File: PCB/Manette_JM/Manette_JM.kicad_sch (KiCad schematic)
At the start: 33 parts, among them J1 Jack 1, J10 Bouton 2, J11 Bouton 3, J12 Bouton 4, J13 DEL PWR, J14 Joystick 0, J15 Jack 7, J16 Jack 8, J2 Jack 3, J3 Jack 4, J4 Jack 5, J5 Jack 6, J6 Jack 2, J7 Jack 0, J8 Bouton 0, J9 Bouton 1, U1 NodeMCU1.0(ESP-12E), U2 ProMicro

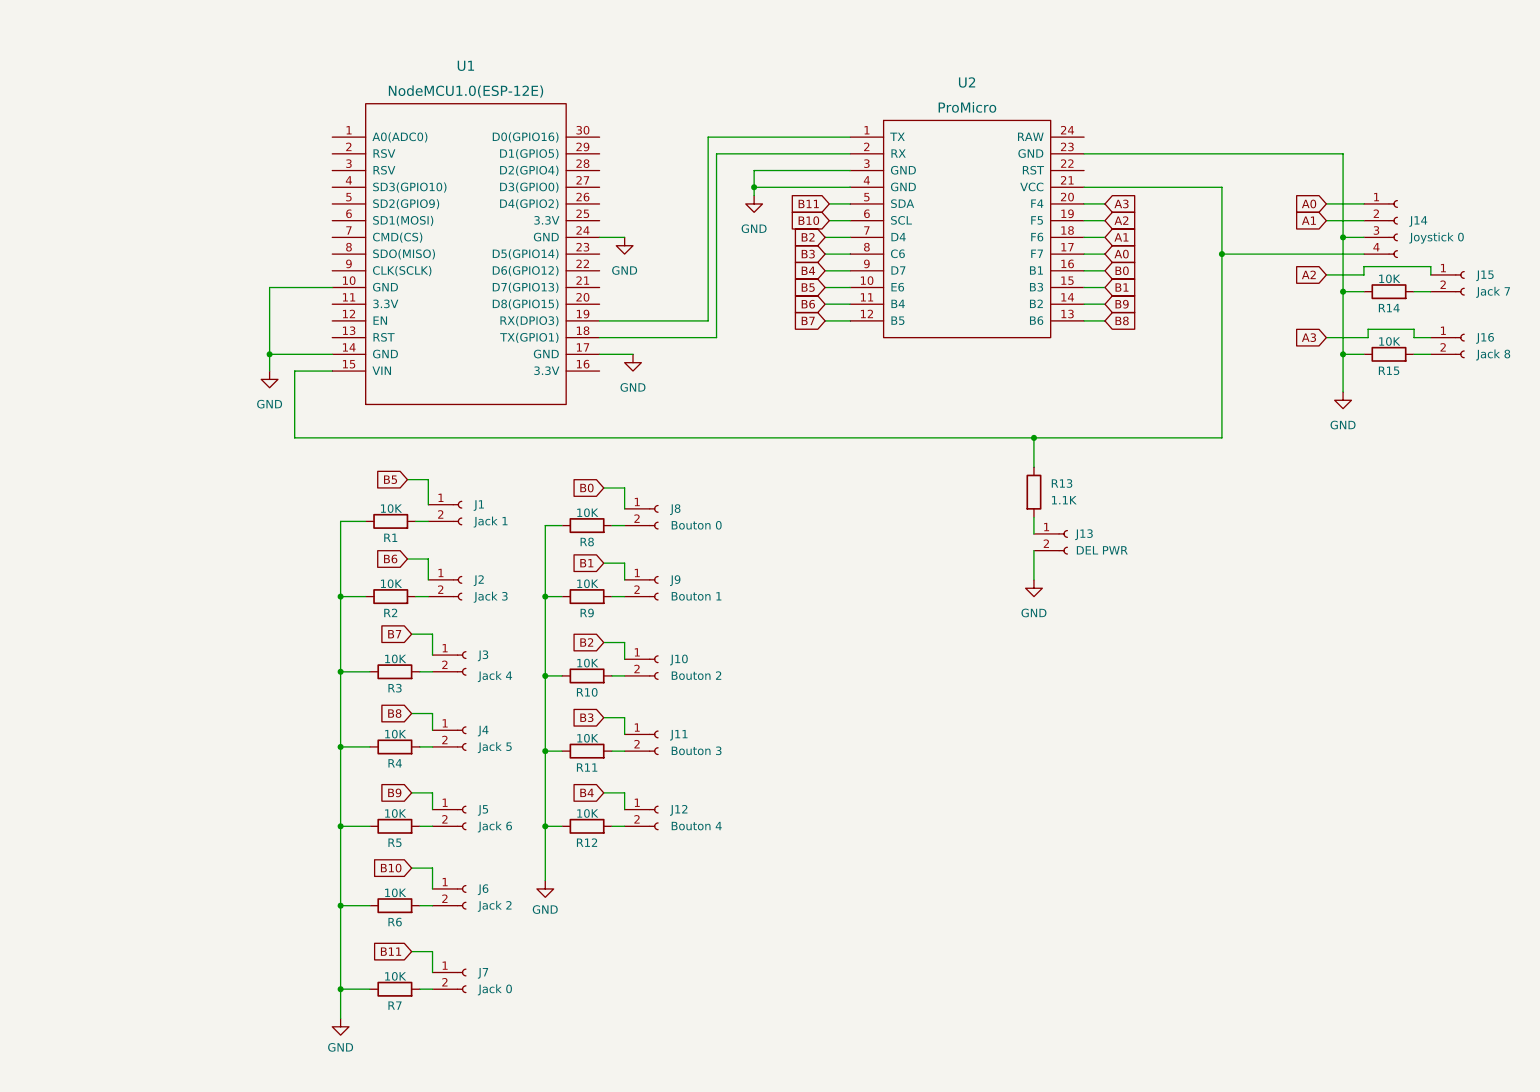
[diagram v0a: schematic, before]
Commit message: Quick changes
modification code et schéma
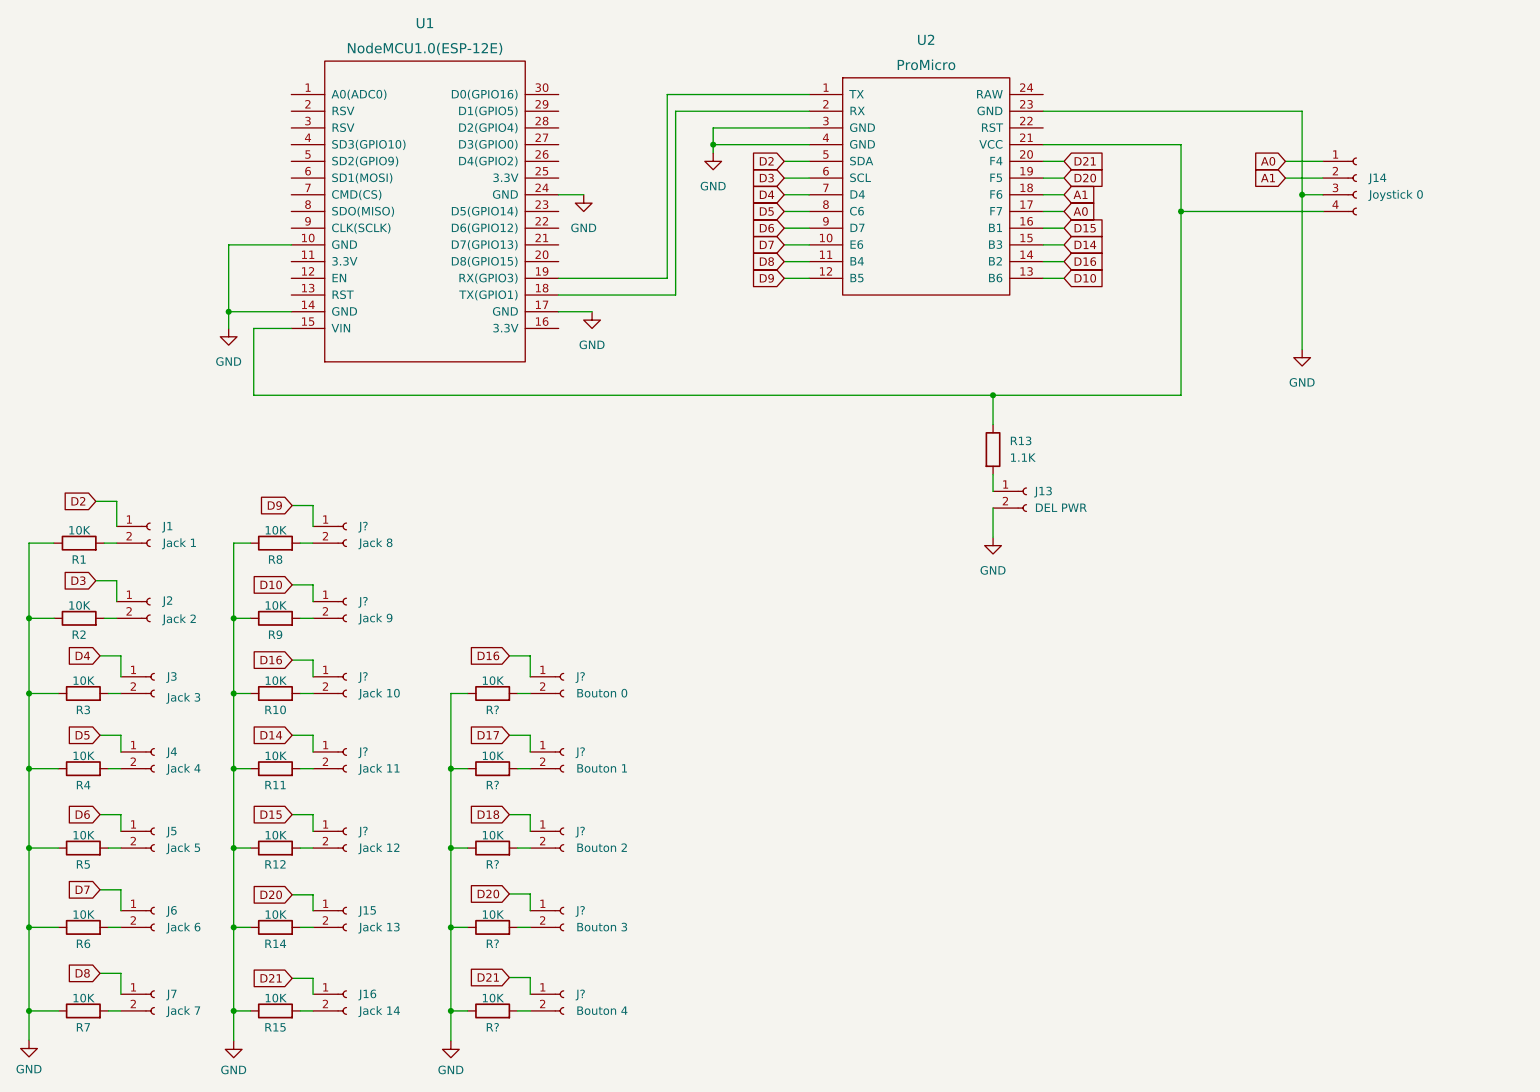
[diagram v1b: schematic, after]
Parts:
- removed J10: Bouton 2, Connector_PinHeader_2.54mm:PinHeader_1x02_P2.54mm_Vertical, symbol Connector:Conn_01x02_Female
- removed J11: Bouton 3, Connector_PinHeader_2.54mm:PinHeader_1x02_P2.54mm_Vertical, symbol Connector:Conn_01x02_Female
- removed J12: Bouton 4, Connector_PinHeader_2.54mm:PinHeader_1x02_P2.54mm_Vertical, symbol Connector:Conn_01x02_Female
- removed J8: Bouton 0, Connector_PinHeader_2.54mm:PinHeader_1x02_P2.54mm_Vertical, symbol Connector:Conn_01x02_Female
- removed J9: Bouton 1, Connector_PinHeader_2.54mm:PinHeader_1x02_P2.54mm_Vertical, symbol Connector:Conn_01x02_Female
- added J?: Bouton 1, Connector_PinHeader_2.54mm:PinHeader_1x02_P2.54mm_Vertical, symbol Connector:Conn_01x02_Female
- added J?: Bouton 4, Connector_PinHeader_2.54mm:PinHeader_1x02_P2.54mm_Vertical, symbol Connector:Conn_01x02_Female
- added J?: Jack 12, Connector_PinHeader_2.54mm:PinHeader_1x02_P2.54mm_Vertical, symbol Connector:Conn_01x02_Female
- added J?: Bouton 0, Connector_PinHeader_2.54mm:PinHeader_1x02_P2.54mm_Vertical, symbol Connector:Conn_01x02_Female
- added J?: Jack 10, Connector_PinHeader_2.54mm:PinHeader_1x02_P2.54mm_Vertical, symbol Connector:Conn_01x02_Female
- added J?: Jack 9, Connector_PinHeader_2.54mm:PinHeader_1x02_P2.54mm_Vertical, symbol Connector:Conn_01x02_Female
- added J?: Jack 11, Connector_PinHeader_2.54mm:PinHeader_1x02_P2.54mm_Vertical, symbol Connector:Conn_01x02_Female
- added J?: Bouton 2, Connector_PinHeader_2.54mm:PinHeader_1x02_P2.54mm_Vertical, symbol Connector:Conn_01x02_Female
- added J?: Jack 8, Connector_PinHeader_2.54mm:PinHeader_1x02_P2.54mm_Vertical, symbol Connector:Conn_01x02_Female
- added J?: Bouton 3, Connector_PinHeader_2.54mm:PinHeader_1x02_P2.54mm_Vertical, symbol Connector:Conn_01x02_Female
- added R? (x5): 10K, Resistor_SMD:R_0805_2012Metric_Pad1.20x1.40mm_HandSolder, symbol Device:R
- J15: value Jack 7 -> Jack 13
- J16: value Jack 8 -> Jack 14
- J2: value Jack 3 -> Jack 2
- J3: value Jack 4 -> Jack 3
- J4: value Jack 5 -> Jack 4
- J5: value Jack 6 -> Jack 5
- J6: value Jack 2 -> Jack 6
- J7: value Jack 0 -> Jack 7
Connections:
- net GND: now also R?.1, R?.1, R?.1, R?.1, R?.1
- net at R10.2: now also J?.2 (Pin_2)
- net at R9.2: now also J?.2 (Pin_2)
- net at R8.2: now also J?.2 (Pin_2)
- net at R12.2: now also J?.2 (Pin_2)
- net at R11.2: now also J?.2 (Pin_2)
- net A2 renamed D20
- net D20: now also J?.1 (Pin_1)
- net A3 renamed D21
- net D21: now also J?.1 (Pin_1)
- net B0 renamed D15
- net D15: now also J?.1 (Pin_1)
- net B1 renamed D14
- net D14: now also J?.1 (Pin_1)
- net B10 renamed D3
- net D3: now also J2.1 (Pin_1); no longer J6.1 (Pin_1)
- net B11 renamed D2
- net D2: now also J1.1 (Pin_1); no longer J7.1 (Pin_1)
- net B2 renamed D4
- net D4: now also J3.1 (Pin_1)
- net B3 renamed D5
- net D5: now also J4.1 (Pin_1)
- net B4 renamed D6
- net D6: now also J5.1 (Pin_1)
- net B5 renamed D7
- net D7: now also J6.1 (Pin_1); no longer J1.1 (Pin_1)
- net B6 renamed D8
- net D8: now also J7.1 (Pin_1); no longer J2.1 (Pin_1)
- net B7 renamed D9
- net D9: now also J?.1 (Pin_1); no longer J3.1 (Pin_1)
- net B8 renamed D10
- net D10: now also J?.1 (Pin_1); no longer J4.1 (Pin_1)
- net B9 renamed D16
- net D16: now also J?.1 (Pin_1), J?.1 (Pin_1); no longer J5.1 (Pin_1)
- new net: J?.2 (Pin_2), R?.2 (x5)
- new net D17: J?.1 (Pin_1)
- new net D18: J?.1 (Pin_1)
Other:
- moved on the sheet: J1, J13, J14, J15, J16, J2, J3, J4, J5, J6, J7, R1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
